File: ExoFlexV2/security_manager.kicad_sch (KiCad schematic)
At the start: 8 parts, among them U10 SN74LV4T08PWR_V2, U11 SN74HC7032D_V2, U7 SN74HC7032D_V2, U8 SN74HC7032D_V2, U9 SN74LV4T08PWR_V2

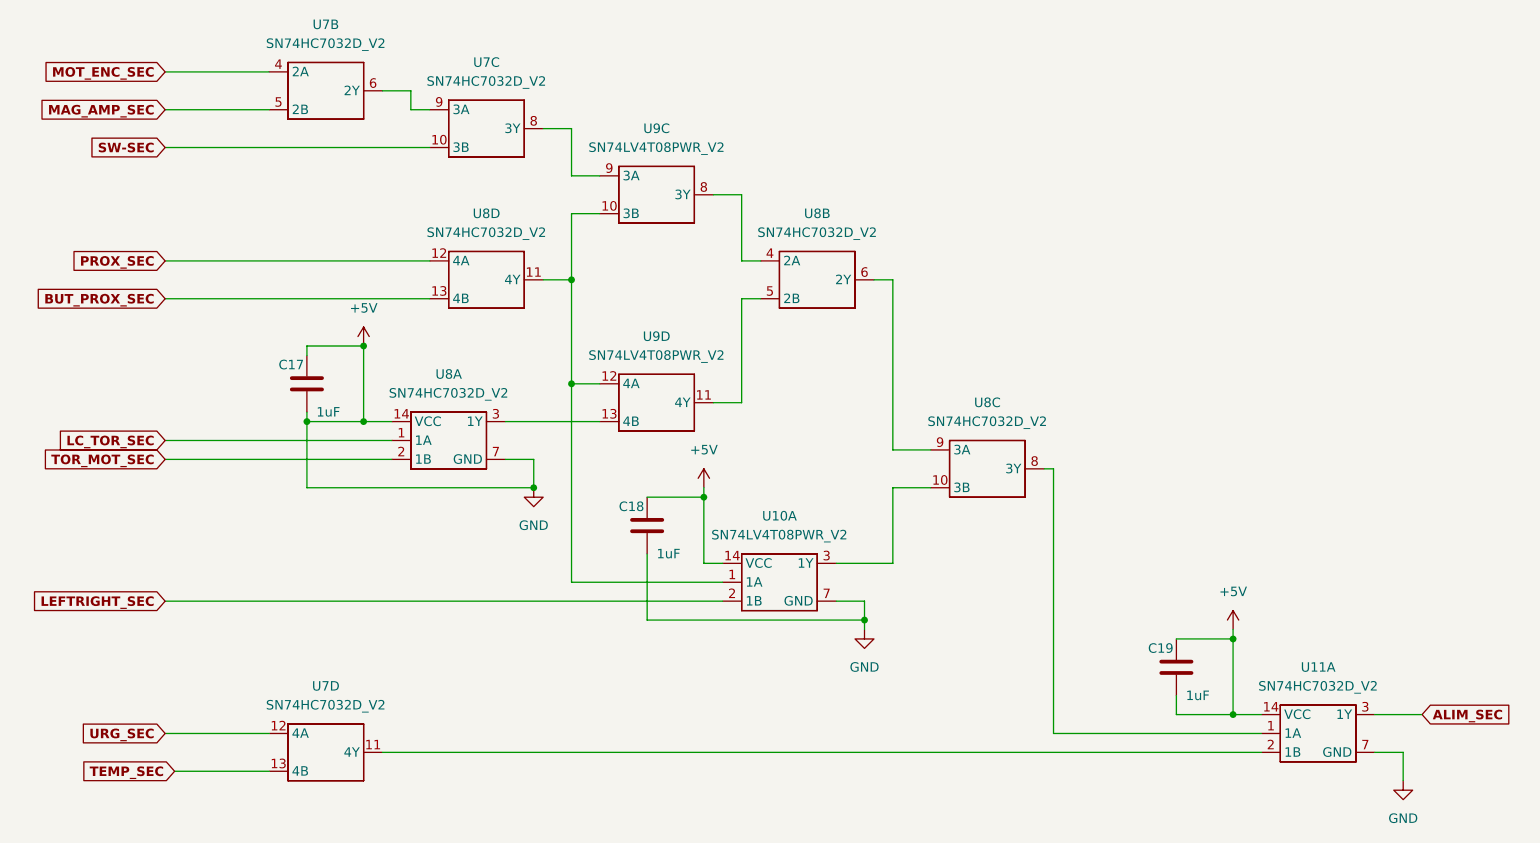
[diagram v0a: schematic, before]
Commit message: Placement
Début du placement et modification d'après dernier review
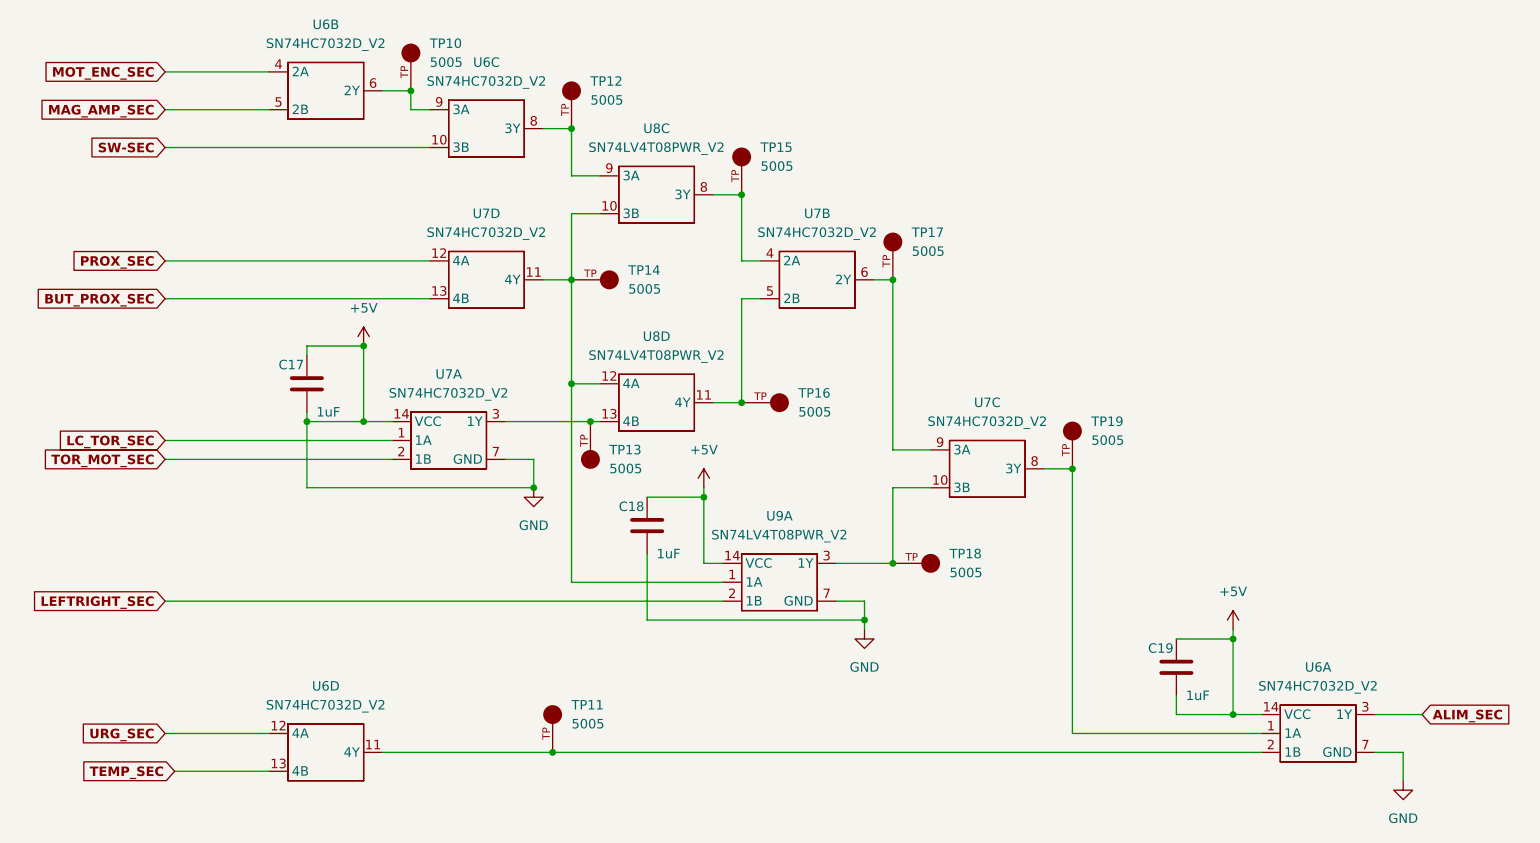
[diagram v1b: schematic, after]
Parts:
- added TP10, TP11, TP12, TP13, TP14, TP15, TP16, TP17, TP18, TP19: 5005, FootPrint:KEYSTONE_5005, symbol SymLib:5005
- renumbered U7 to U6, U11 to U6, U8 to U7, U9 to U8, U10 to U9
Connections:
- net at U6.6 (2Y), U6.9 (3A): now also TP10.TP
- net at U7.10 (3B), U9.3 (1Y): now also TP18.TP
- net at U6.1 (1A), U7.8 (3Y): now also TP19.TP
- net at U7.6 (2Y), U7.9 (3A): now also TP17.TP
- net at U6.11 (4Y), U6.2 (1B): now also TP11.TP
- net at U7.11 (4Y), U8.10 (3B), U8.12 (4A)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: now also TP14.TP
- net at U7.4 (2A), U8.8 (3Y): now also TP15.TP
- net at U6.8 (3Y), U8.9 (3A): now also TP12.TP
- net at U7.5 (2B), U8.11 (4Y): now also TP16.TP
- net at U7.3 (1Y), U8.13 (4B): now also TP13.TP
